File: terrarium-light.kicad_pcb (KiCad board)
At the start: 2 copper layers, 100 x 100 mm, 50 parts, among them J2 USB_C_Receptacle_USB2.0_16P, Q1 UMH3N, U1 CH340C, U2 TPS61169DCKR, U3 TPS61169DCKR, U4 LM1117S-3.3, U5 ESP32-S3-MINI-1U

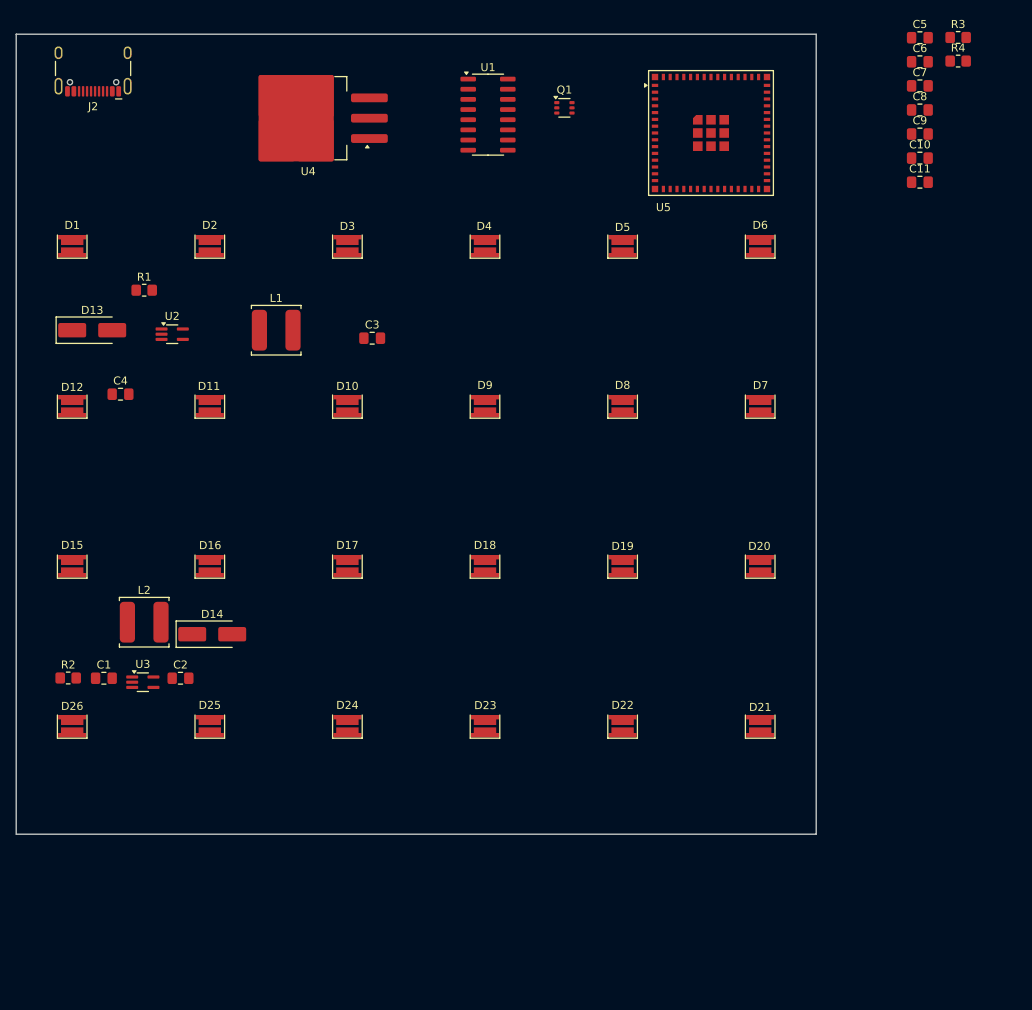
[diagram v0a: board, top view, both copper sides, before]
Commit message: more stuff
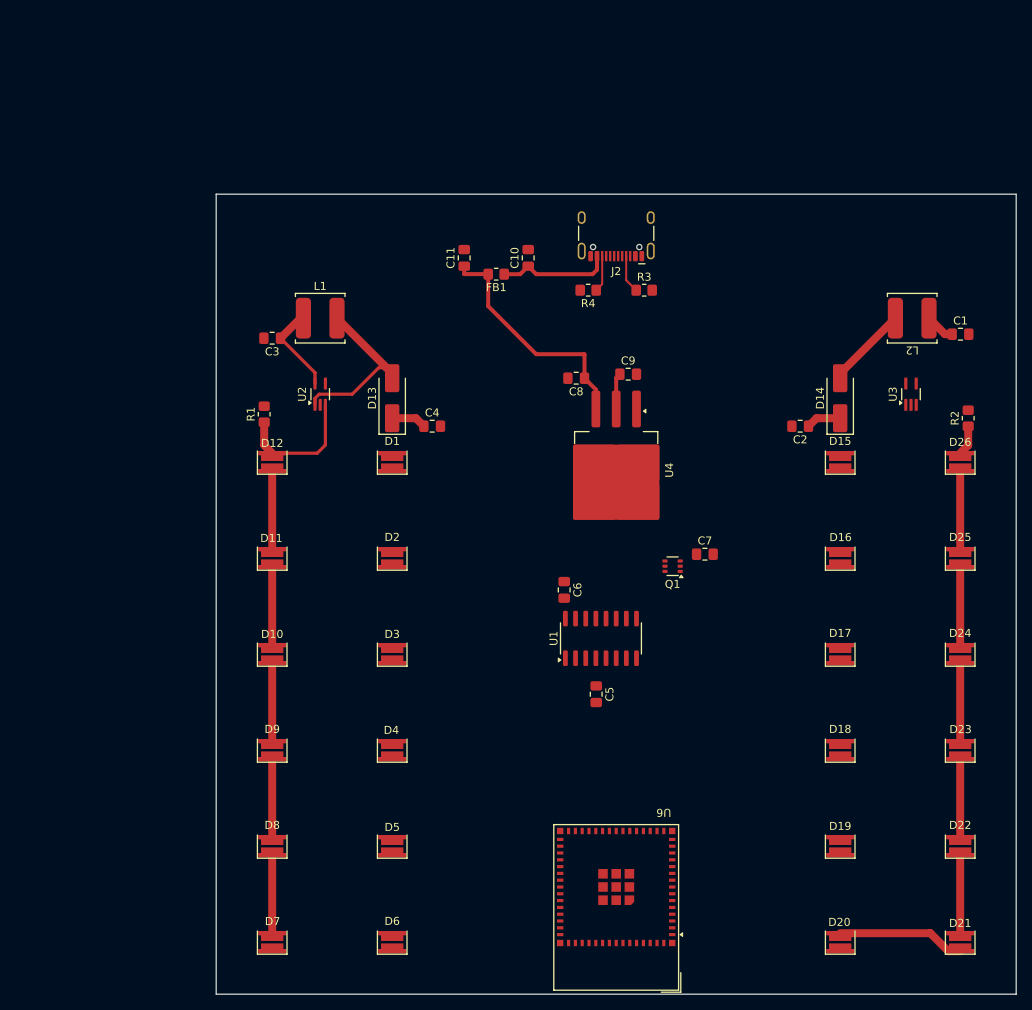
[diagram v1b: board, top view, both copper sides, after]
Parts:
- removed U5: ESP32-S3-MINI-1U, RF_Module:ESP32-S2-MINI-1U
- added FB1: MI0805K400R-10, Resistor_SMD:R_0805_2012Metric_Pad1.20x1.40mm_HandSolder, F.Cu at (85.0, 60.0)
- added U6: ESP32-S3-MINI-1, RF_Module:ESP32-S2-MINI-1, F.Cu at (100.0, 139.2)
- moved R2 117.1 mm to (144.0, 78.0), turned to 90 degrees
- moved D26 115.8 mm to (143.0, 83.5)
- moved C1 115.4 mm to (143.0, 67.5)
- moved L2 103.2 mm to (137.0, 65.5), turned to 180 degrees
- moved U3 102.5 mm to (136.8, 75.0), turned to 90 degrees
- moved D6 98.4 mm to (72.0, 143.5)
- moved D15 96.9 mm to (128.0, 83.5)
- moved D25 96.1 mm to (143.0, 95.5)
- moved C5 91.5 mm to (97.5, 112.5), turned to -90 degrees
- moved D7 90.6 mm to (57.0, 143.5)
- moved D14 83.9 mm to (128.0, 75.5), turned to 90 degrees
- moved C2 83.6 mm to (123.0, 79.0), turned to 180 degrees
- moved D5 80.3 mm to (72.0, 131.5)
- moved C6 79.6 mm to (93.5, 99.5), turned to -90 degrees
- moved D16 78.8 mm to (128.0, 95.5)
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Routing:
- net +5V: track 0.00 -> 48.0 mm
- net Net-(D13-A): track 0.00 -> 21.7 mm
- net Net-(D12-K): track 0.00 -> 16.4 mm
- net Net-(D20-K): track 0.00 -> 15.9 mm
- net VBUS: track 0.00 -> 14.4 mm
- net Net-(D14-A): track 0.00 -> 10.4 mm
- net Net-(D8-K): track 0.00 -> 9.75 mm
- net Net-(D7-K): track 0.00 -> 9.75 mm
- net Net-(D25-K): track 0.00 -> 9.75 mm
- net Net-(D24-K): track 0.00 -> 9.75 mm
- net Net-(D23-K): track 0.00 -> 9.75 mm
- net Net-(D22-K): track 0.00 -> 9.75 mm
- net Net-(D21-K): track 0.00 -> 9.75 mm
- net Net-(D11-K): track 0.00 -> 9.75 mm
- net Net-(D10-K): track 0.00 -> 9.75 mm
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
